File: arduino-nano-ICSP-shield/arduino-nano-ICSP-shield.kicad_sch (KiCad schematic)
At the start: 2 parts, among them J1 Analog, J2 Digital

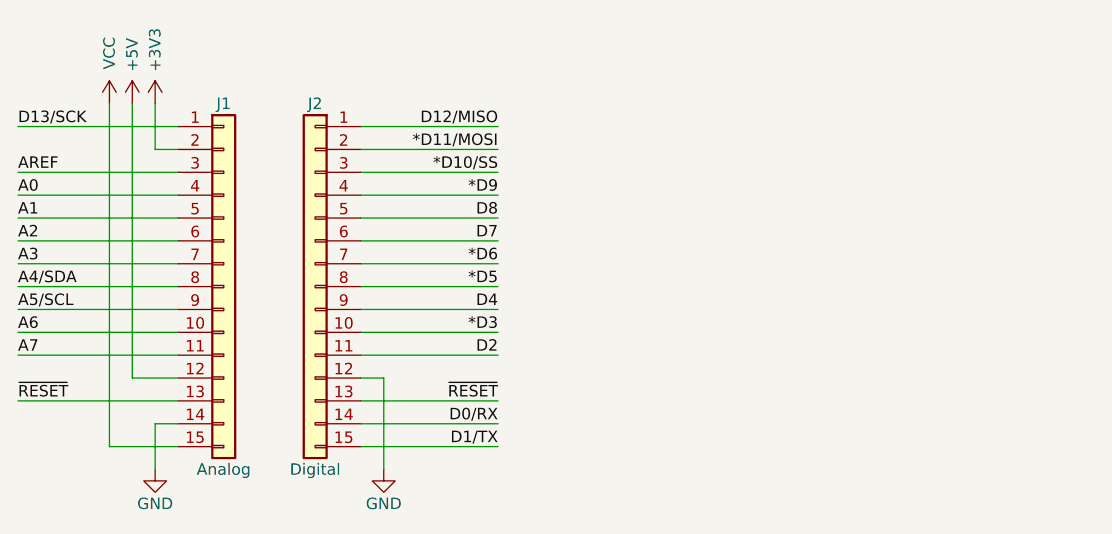
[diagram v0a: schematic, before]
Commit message: init led's
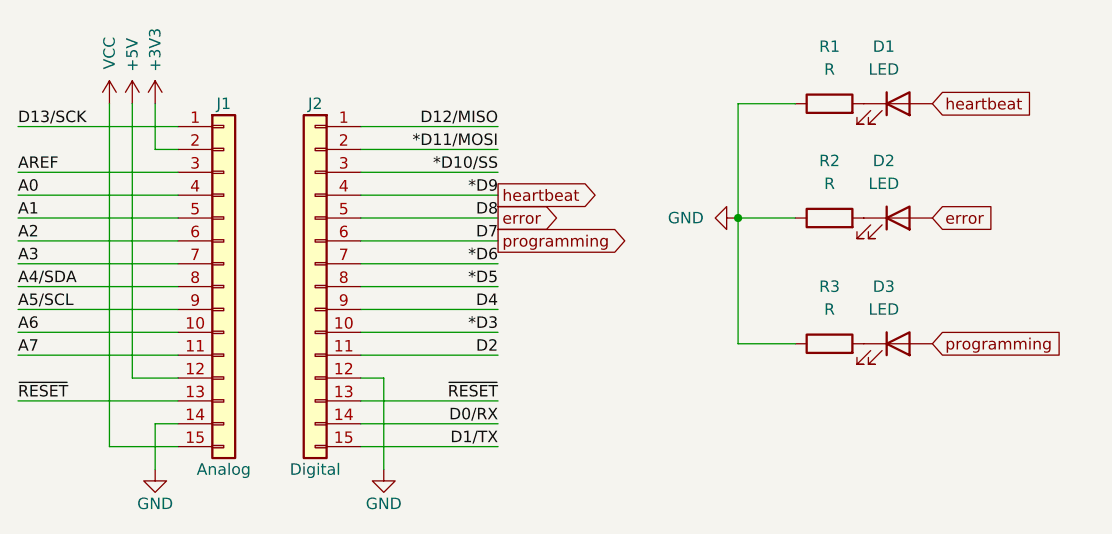
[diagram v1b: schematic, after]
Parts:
- added D1, D2, D3: LED, LED_SMD:LED_0805_2012Metric_Pad1.15x1.40mm_HandSolder, symbol Device:LED
- added R1, R2, R3: R, Resistor_SMD:R_0805_2012Metric_Pad1.20x1.40mm_HandSolder, symbol Device:R
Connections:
- net GND: now also R1.1, R2.1, R3.1
- net *D9 renamed heartbeat
- net heartbeat: now also D1.2 (A)
- net D7 renamed programming
- net programming: now also D3.2 (A)
- net D8 renamed error
- net error: now also D2.2 (A)
- new net: D2.1 (K), R2.2
- new net: D3.1 (K), R3.2
- new net: D1.1 (K), R1.2
